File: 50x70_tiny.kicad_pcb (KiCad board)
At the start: 2 copper layers, 78.2 x 78.5 mm, 20 parts, among them J1 Barrel_Jack_MountingPin, J2 Conn_01x04_F, J3 Conn_02x03_M, Q1 Q_NMOS_GDS, SW1 SW_MEC_5E, SW2 SW_MEC_5E, U1 ATtiny85, U2 L78L05_TO92

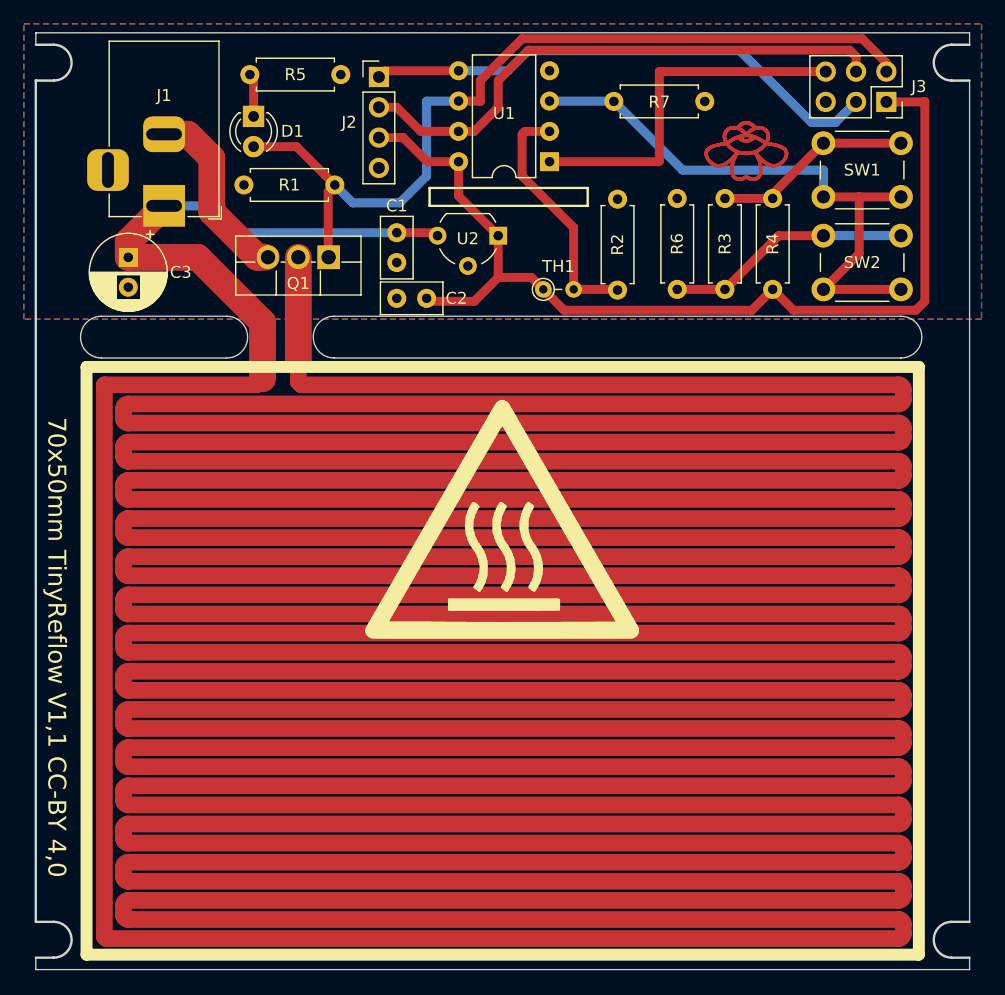
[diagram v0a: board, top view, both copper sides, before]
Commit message: redesign, 3D models and a picture
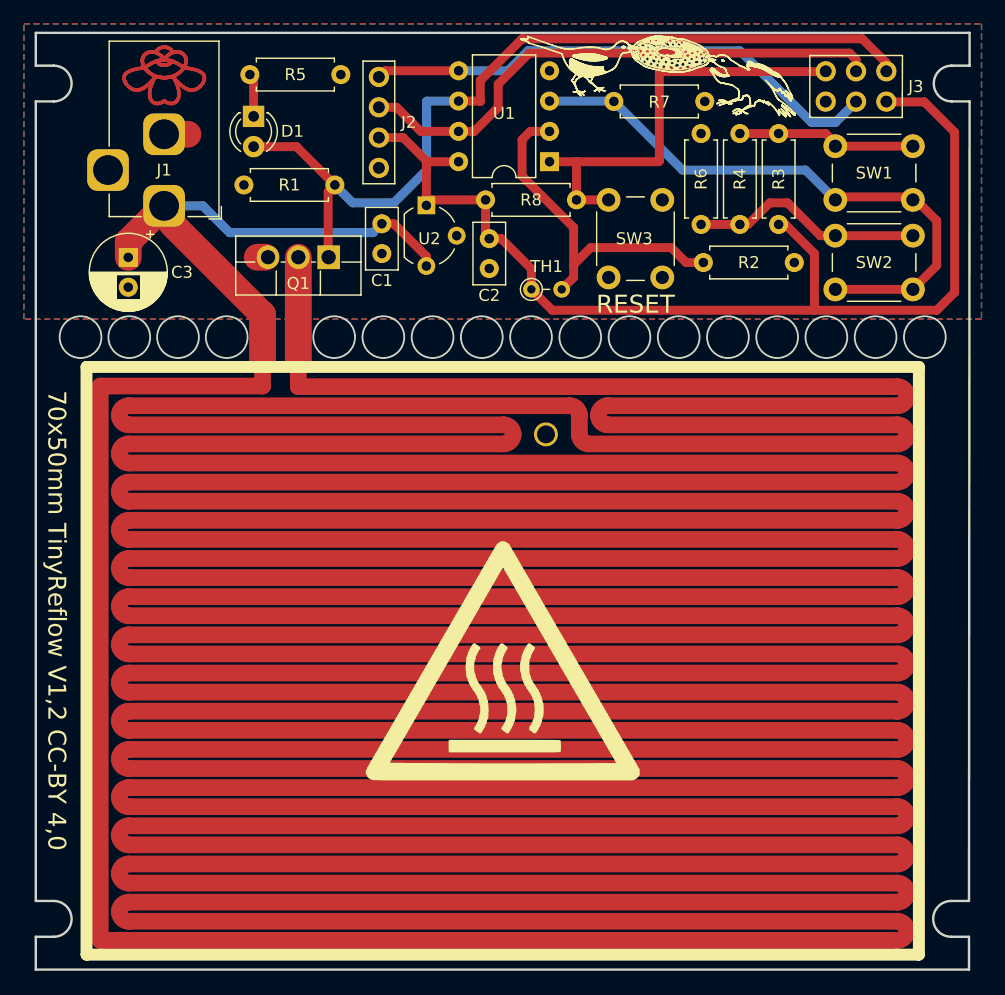
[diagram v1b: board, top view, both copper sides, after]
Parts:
- added ?: , , F.Cu at (149.5, 103.7)
- added R8: 10kΩ, Resistor_THT:R_Axial_DIN0207_L6.3mm_D2.5mm_P7.62mm_Horizontal, F.Cu at (152.1, 84.0)
- added SW3: SW_MEC_5E, Button_Switch_THT:SW_PUSH_6mm_H4.3mm, F.Cu at (154.8, 90.5)
- J2: footprint Connector_PinHeader_2.54mm:PinHeader_1x04_P2.54mm_Vertical -> Connector_PinSocket_2.54mm:PinSocket_1x04_P2.54mm_Vertical
- J3: footprint Connector_PinSocket_2.54mm:PinSocket_2x03_P2.54mm_Vertical -> Connector_PinHeader_2.54mm:PinHeader_2x03_P2.54mm_Vertical
- moved R2 7.55 mm to (162.7, 89.2), turned to 0 degrees
- moved C2 7.25 mm to (144.8, 87.2), turned to -90 degrees
- moved U2 6.53 mm to (139.5, 84.5), turned to -90 degrees
- moved R6 5.80 mm to (162.5, 86.1)
- moved R4 5.58 mm to (165.8, 78.4)
- moved R3 5.46 mm to (169.0, 86.1)
- moved J3 2.57 mm to (178.0, 73.2)
- moved C1 1.46 mm to (135.8, 86.0)
- moved SW1 1.03 mm to (180.2, 84.0)
- moved SW2 1.00 mm to (180.2, 91.5)
- moved TH1 1.00 mm to (148.3, 91.5)
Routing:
- net GND: track 15.4 -> 2.69 mm
- net Net-(R2-Pad1): track 20.9 -> 29.5 mm
- net +5V: track 84.1 -> 91.8 mm
- net Net-(J3-Pad6): track 30.7 -> 35.9 mm
- net Net-(R3-Pad2): track 16.9 -> 15.0 mm
- net Net-(R4-Pad2): track 20.6 -> 18.9 mm
- net VCC: track 2100.8 -> 2099.5 mm
- net Net-(D1-Pad2): track 73.3 -> 72.7 mm
- net Net-(J2-Pad2): track 46.4 -> 45.9 mm
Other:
- outline, holes or cut-outs redrawn
- board text added: "70x50mm TinyReflow V1,2 CC-BY 4,0"
- board text added: "RESET"
- board text removed: "70x50mm TinyReflow V1,1 CC-BY 4,0"
